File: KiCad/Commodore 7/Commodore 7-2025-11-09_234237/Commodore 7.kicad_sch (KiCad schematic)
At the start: 1 part, among them J2 Conn_02x20_Odd_Even_MountingP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

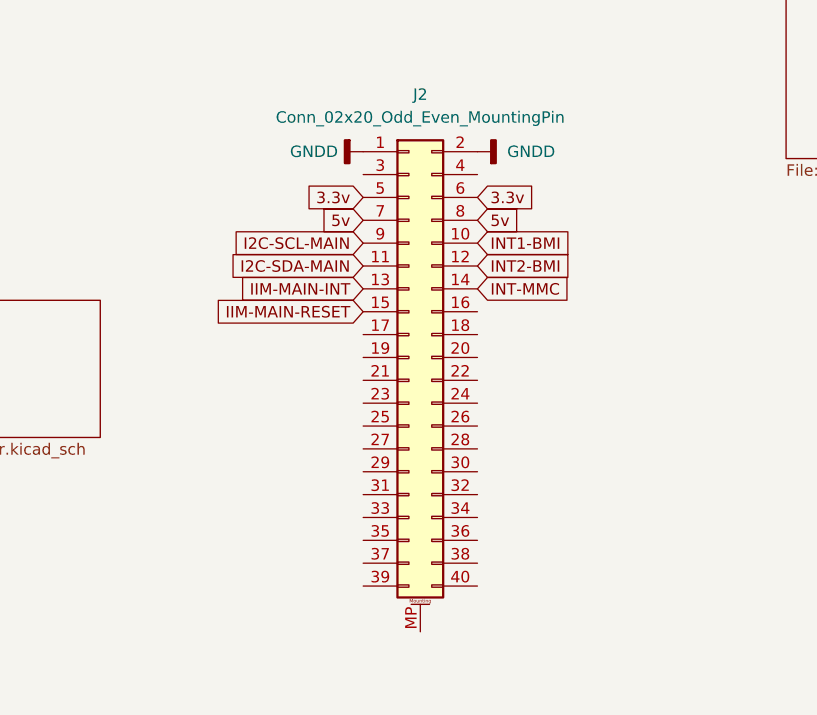
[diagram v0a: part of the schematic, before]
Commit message: updated some labels idk
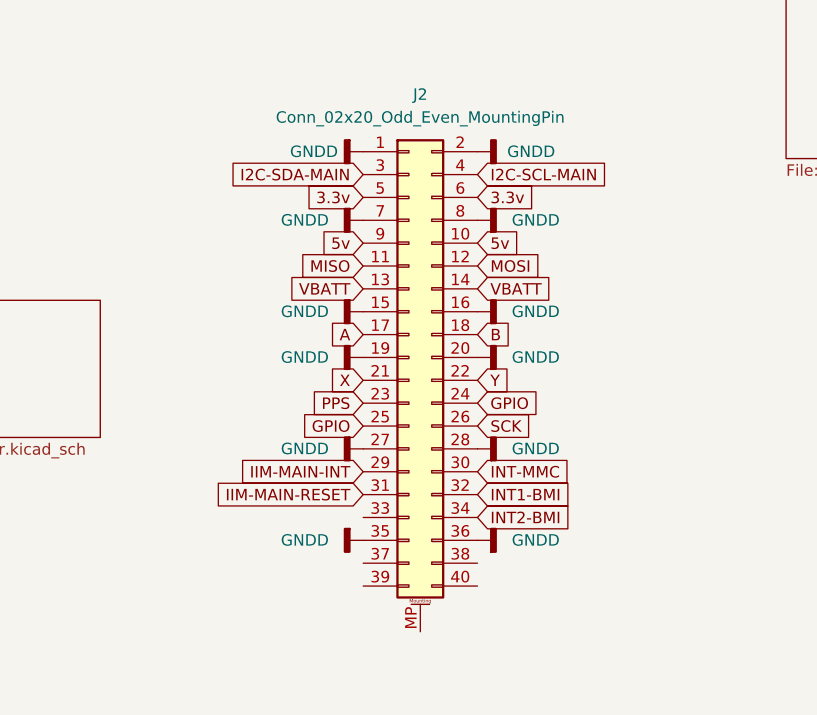
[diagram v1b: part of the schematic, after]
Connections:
- net 5v: now also J2.10 (Pin_10), J2.9 (Pin_9); no longer J2.7 (Pin_7), J2.8 (Pin_8)
- net GNDD: now also J2.15 (Pin_15), J2.16 (Pin_16), J2.19 (Pin_19), J2.20 (Pin_20), J2.27 (Pin_27), J2.28 (Pin_28), J2.35 (Pin_35), J2.36 (Pin_36), J2.7 (Pin_7), J2.8 (Pin_8)
- net I2C-SCL-MAIN: now also J2.4 (Pin_4); no longer J2.9 (Pin_9)
- net I2C-SDA-MAIN: now also J2.3 (Pin_3); no longer J2.11 (Pin_11)
- net IIM-MAIN-INT: now also J2.29 (Pin_29); no longer J2.13 (Pin_13)
- net IIM-MAIN-RESET: now also J2.31 (Pin_31); no longer J2.15 (Pin_15)
- net INT-MMC: now also J2.30 (Pin_30); no longer J2.14 (Pin_14)
- net INT1-BMI: now also J2.32 (Pin_32); no longer J2.10 (Pin_10)
- net INT2-BMI: now also J2.34 (Pin_34); no longer J2.12 (Pin_12)
- net A: now reaches J2.17 (Pin_17)
- net B: now reaches J2.18 (Pin_18)
- net X: now reaches J2.21 (Pin_21)
- net Y: now reaches J2.22 (Pin_22)
- net PPS: now reaches J2.23 (Pin_23)
- net GPIO: now reaches J2.24 (Pin_24)
- net GPIO: now also J2.25 (Pin_25)
- net SCK: now reaches J2.26 (Pin_26)
- new net MISO: J2.11 (Pin_11)
- new net MOSI: J2.12 (Pin_12)
- new net VBATT: J2.13 (Pin_13), J2.14 (Pin_14)
